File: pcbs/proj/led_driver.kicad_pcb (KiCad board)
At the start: 4 copper layers, 100 x 82.5 mm, 348 parts, among them J1 Conn_02x32_Counter_Clockwise, J2 Conn_02x03_Odd_Even, J3 Conn_01x05, J4 Conn_02x05_Odd_Even, J5 Barrel_Jack, J6 Conn_02x19_Odd_Even, J7 Conn_02x19_Odd_Even, J8 Conn_01x07, Q1 MBT3904DW1, Q10 MBT3904DW1, Q11 MBT3904DW1, Q12 MBT3904DW1, Q13 MBT3904DW1, Q14 MBT3904DW1, Q15 MBT3904DW1, Q16 MBT3904DW1, Q17 MBT3904DW1, Q18 MBT3904DW1, Q19 MBT3904DW1, Q2 MBT3904DW1, Q20 MBT3904DW1, Q21 MBT3904DW1, Q22 MBT3904DW1, Q23 MBT3904DW1, Q24 MBT3904DW1, Q25 MBT3904DW1, Q26 MBT3904DW1, Q27 MBT3904DW1, Q28 MBT3904DW1, Q29 MBT3904DW1, Q3 MBT3904DW1, Q30 MBT3904DW1, Q31 MBT3904DW1, Q32 MBT3904DW1, Q4 MBT3904DW1, Q5 MBT3904DW1, Q6 MBT3904DW1, Q7 MBT3904DW1, Q8 MBT3904DW1, Q9 MBT3904DW1, SW1 MY_SW_Push_Dual, SW2 Rotary_Encoder, SW3 Rotary_Encoder, U1 LM324QT, U10 LM324QT, U11 LM324QT, U12 LM324QT, U13 LM324QT, U14 LM324QT, U15 LM324QT, U16 LM324QT, U17 LM324QT, U18 LM324QT, U19 LM324QT, U2 LM324QT, U20 LM324QT, U21 LM324QT, U22 LM324QT, U23 LM324QT, U24 LM324QT, U25 LM324QT, U26 LM324QT, U27 LM324QT, U28 LM324QT, U29 LM324QT, U3 LM324QT, U30 LM324QT, U31 LM324QT, U32 LM324QT, U33 DAC101C085, U34 TS30011/12/13, U4 LM324QT, U5 LM324QT, U6 LM324QT, U7 LM324QT, U8 LM324QT, U9 LM324QT

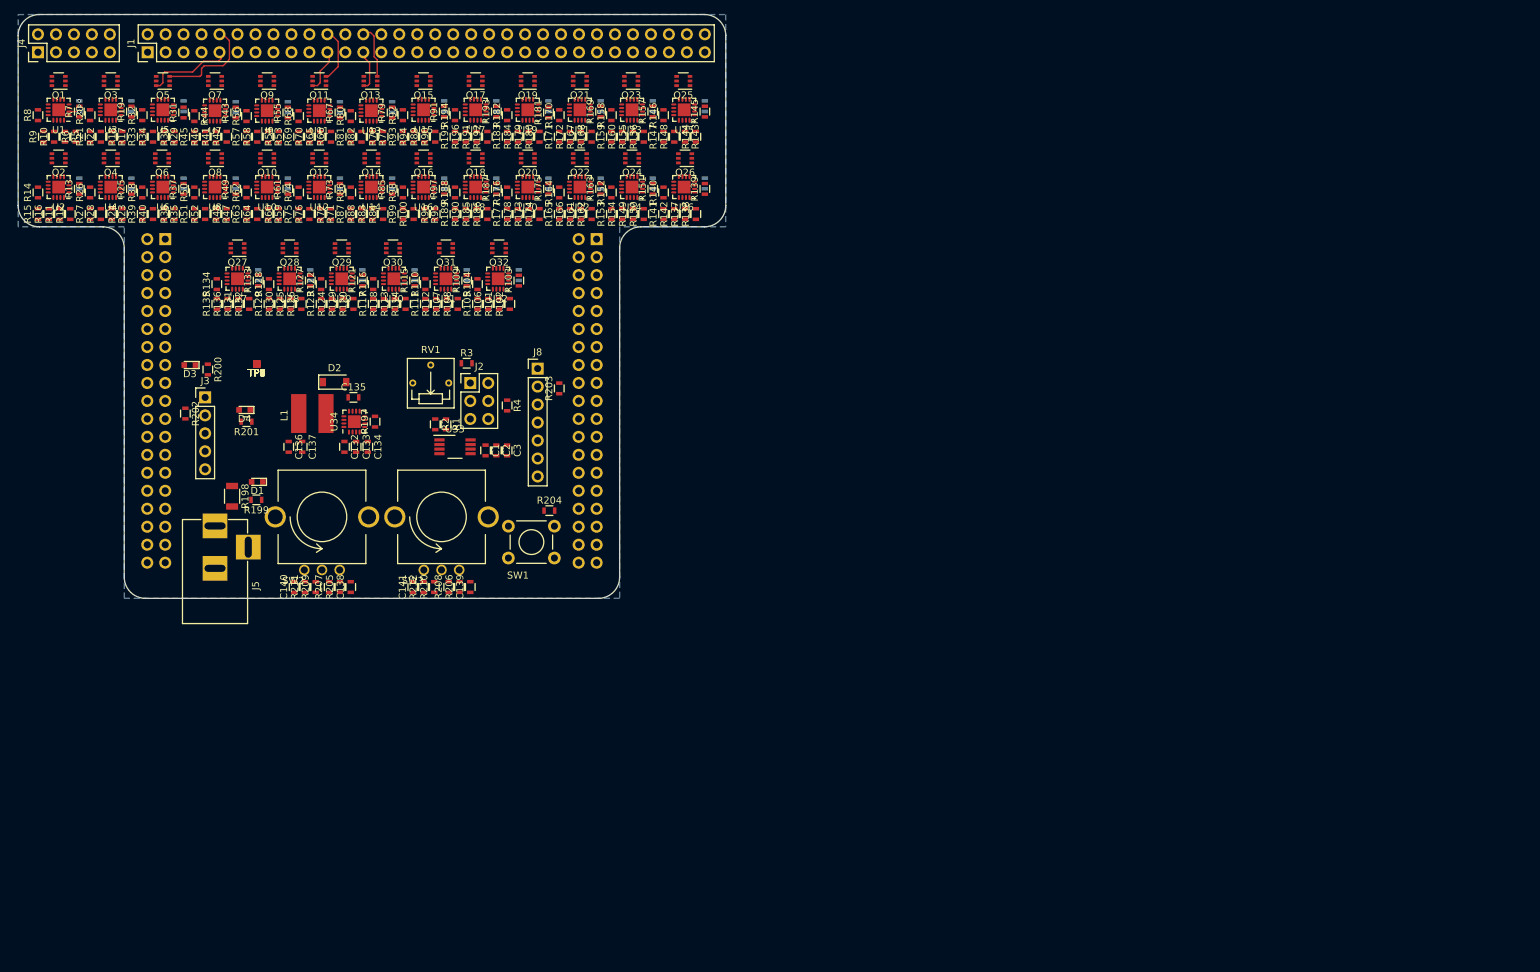
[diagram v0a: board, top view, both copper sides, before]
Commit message: Some progress layouting the beast today.
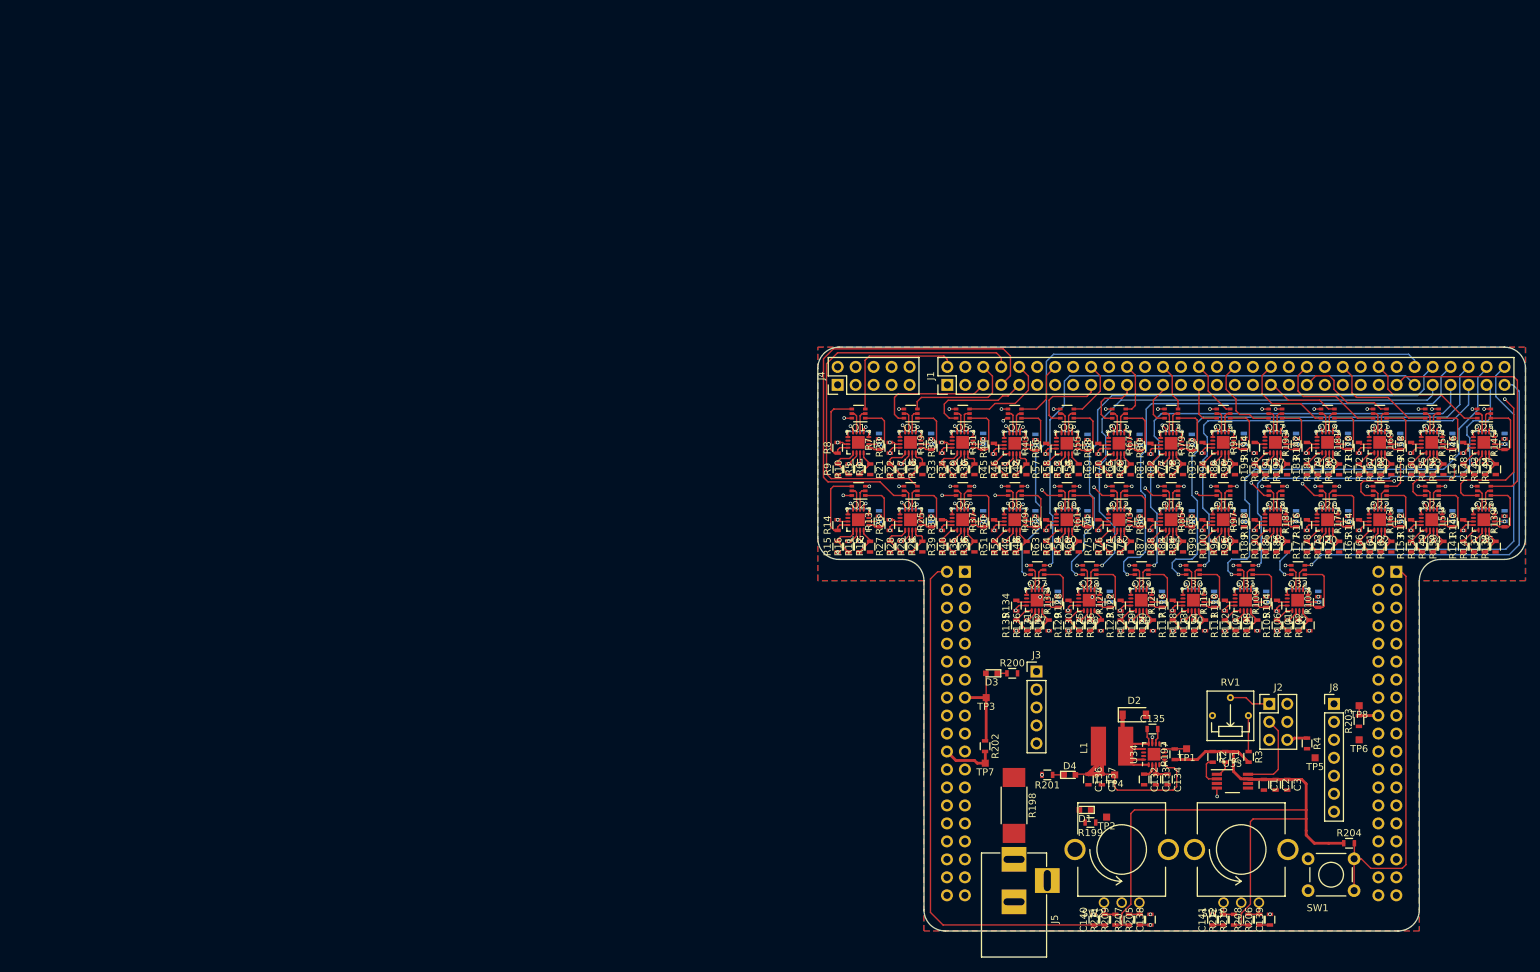
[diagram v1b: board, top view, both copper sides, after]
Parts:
- R198: footprint Resistors_SMD:R_1206 -> Resistors_SMD:R_2512_HandSoldering
- moved TP6 164.6 mm to (174.5, 102.5)
- moved TP8 163.1 mm to (174.5, 97.7)
- moved TP5 159.6 mm to (168.3, 105.0)
- moved TP1 142.2 mm to (150.1, 103.8)
- moved TP2 136.1 mm to (138.8, 113.4)
- moved TP4 134.4 mm to (140.0, 107.4)
- moved D4 127.5 mm to (133.6, 107.4), turned to 0 degrees
- moved R199 126.4 mm to (136.5, 114.2)
- moved D1 125.8 mm to (135.8, 112.4)
- moved R3 123.7 mm to (158.9, 104.9), turned to 270 degrees
- moved J3 123.7 mm to (128.9, 92.8)
- moved R201 123.7 mm to (130.4, 107.4)
- moved R4 122.7 mm to (167.1, 103.0)
- moved Q13 122.5 mm to (148.0, 56.4)
- moved Q25 122.5 mm to (192.2, 56.4)
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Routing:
- net VSIG: track 0.00 -> 281.9 mm, vias 0 -> 64
- net +3V3: track 0.00 -> 119.8 mm
- net PC9: track 0.00 -> 91.6 mm, vias 0 -> 1
- net LED_N_54: track 0.00 -> 86.9 mm, vias 0 -> 1
- net LED_N_53: track 0.00 -> 78.4 mm, vias 0 -> 1
- net LED_N_56: track 0.00 -> 77.5 mm, vias 0 -> 1
- net PC10: track 0.00 -> 75.2 mm
- net LED_N_58: track 0.00 -> 74.5 mm, vias 0 -> 1
- net LED_N_55: track 0.00 -> 73.3 mm, vias 0 -> 1
- net LED_N_60: track 0.00 -> 70.3 mm, vias 0 -> 1
- net LED_N_57: track 0.00 -> 68.2 mm, vias 0 -> 1
- net LED_N_64: track 0.00 -> 63.5 mm, vias 0 -> 1
- net LED_N_62: track 0.00 -> 63.2 mm, vias 0 -> 1
- net LED_N_59: track 0.00 -> 63.1 mm, vias 0 -> 1
- net LED_N_07: track 0.00 -> 61.2 mm
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- added copper zone on F.Cu, net GND
- added copper zone on S2.Cu, net GND
- removed copper zone on GND.Cu, net GND
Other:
- net class Default: clearance 0.15 -> 0.19
- rule trace_clearance: 0.15 -> 0.19
